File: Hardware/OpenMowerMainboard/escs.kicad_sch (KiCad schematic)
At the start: 3 parts, among them U4 xESC2, U5 xESC2, U6 xESC2

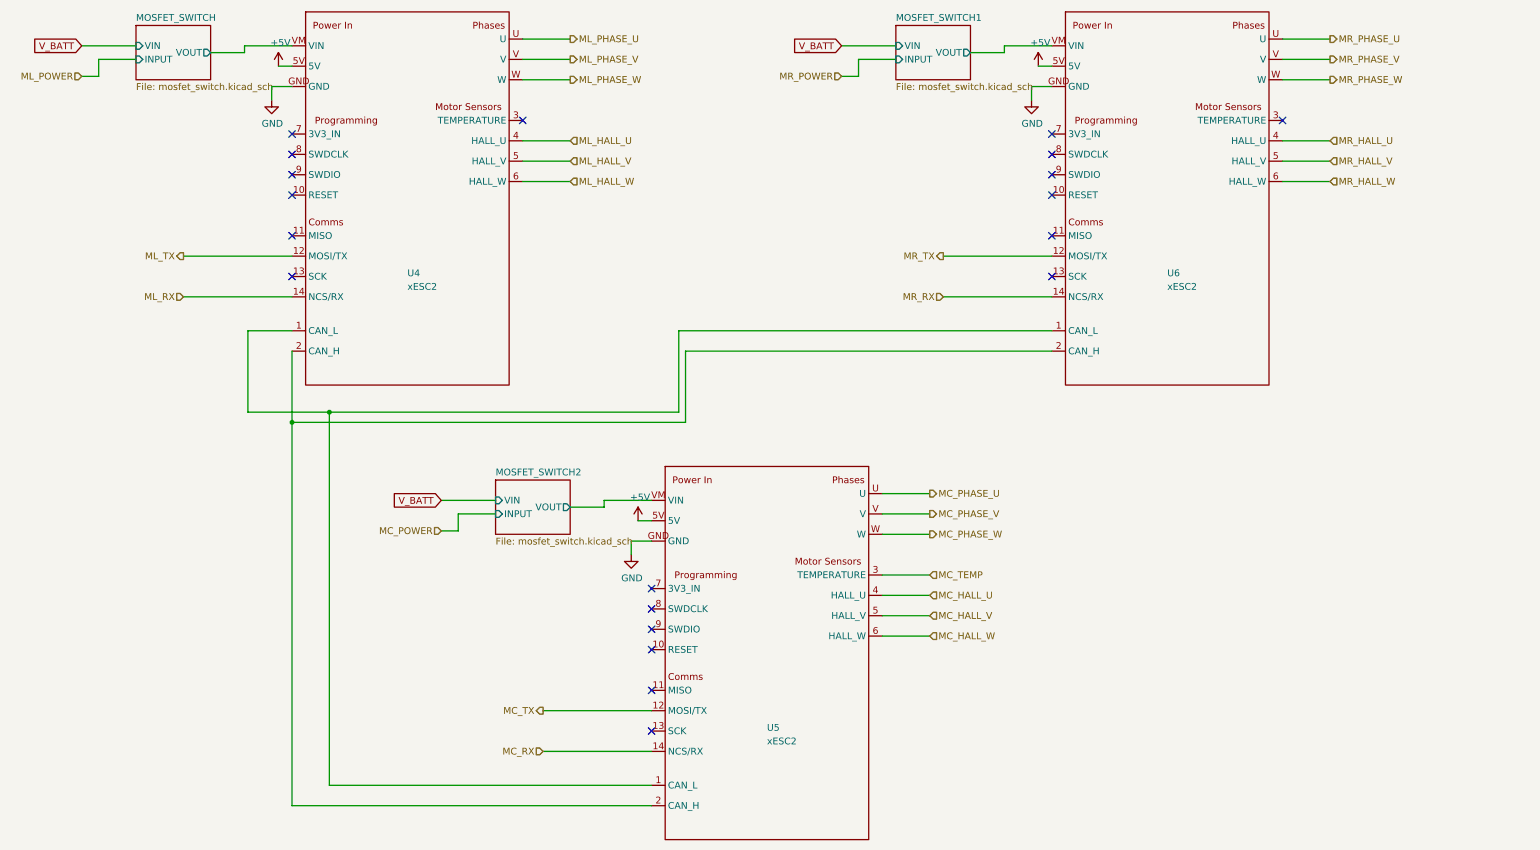
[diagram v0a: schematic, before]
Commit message: wip schematic
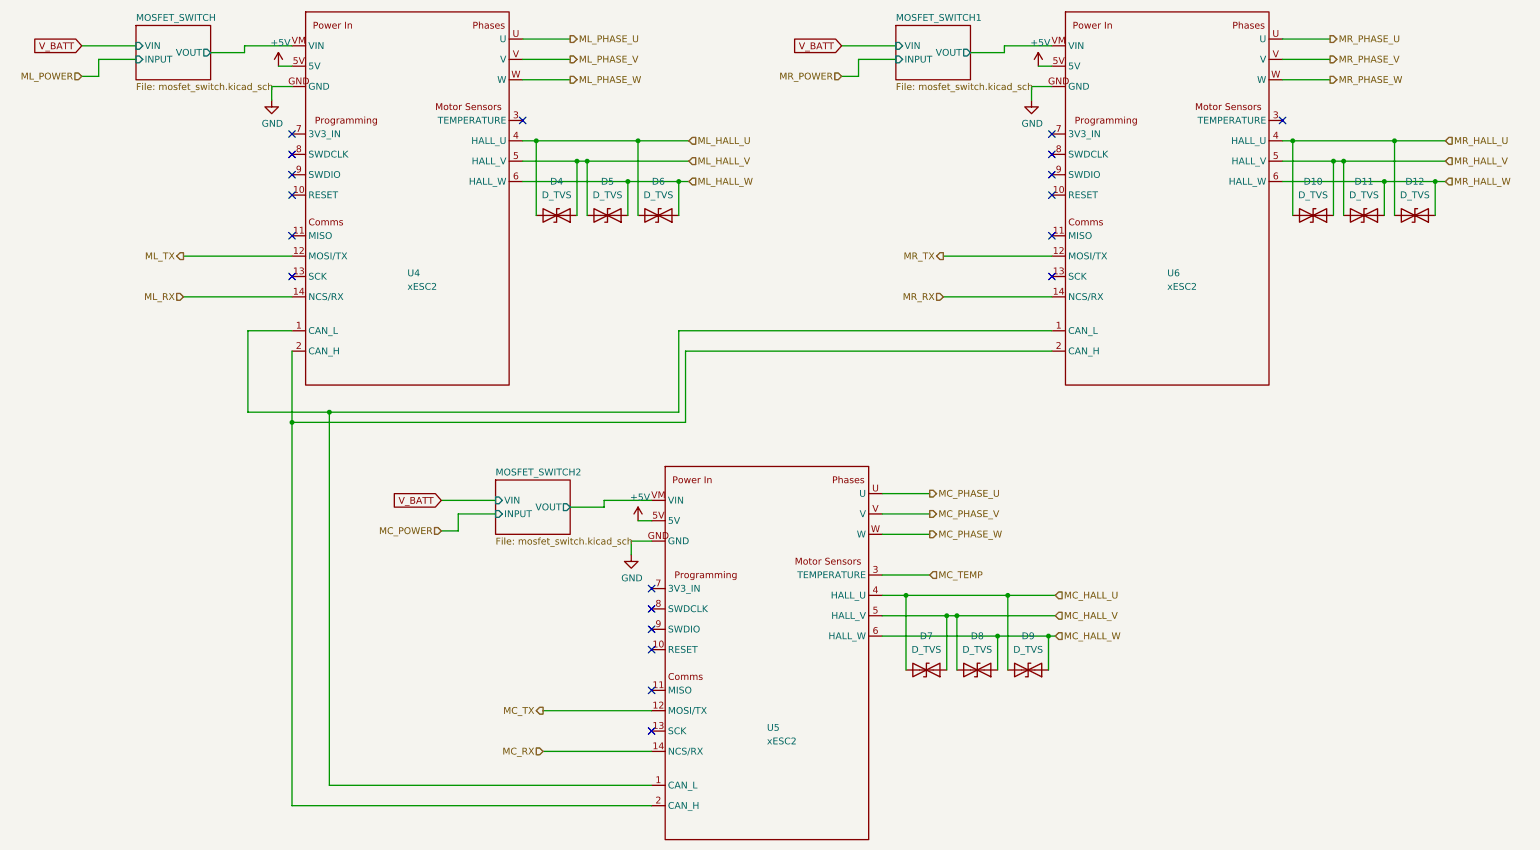
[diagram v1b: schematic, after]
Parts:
- added D10, D11, D12, D4, D5, D6, D7, D8, D9: D_TVS, Diode_SMD:D_SMB, symbol Device:D_TVS
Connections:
- net MC_HALL_U: now also D7.2 (A2), D9.2 (A2)
- net MC_HALL_V: now also D7.1 (A1), D8.2 (A2)
- net MC_HALL_W: now also D8.1 (A1), D9.1 (A1)
- net ML_HALL_U: now also D4.2 (A2), D6.2 (A2)
- net ML_HALL_V: now also D4.1 (A1), D5.2 (A2)
- net ML_HALL_W: now also D5.1 (A1), D6.1 (A1)
- net MR_HALL_U: now also D10.2 (A2), D12.2 (A2)
- net MR_HALL_V: now also D10.1 (A1), D11.2 (A2)
- net MR_HALL_W: now also D11.1 (A1), D12.1 (A1)

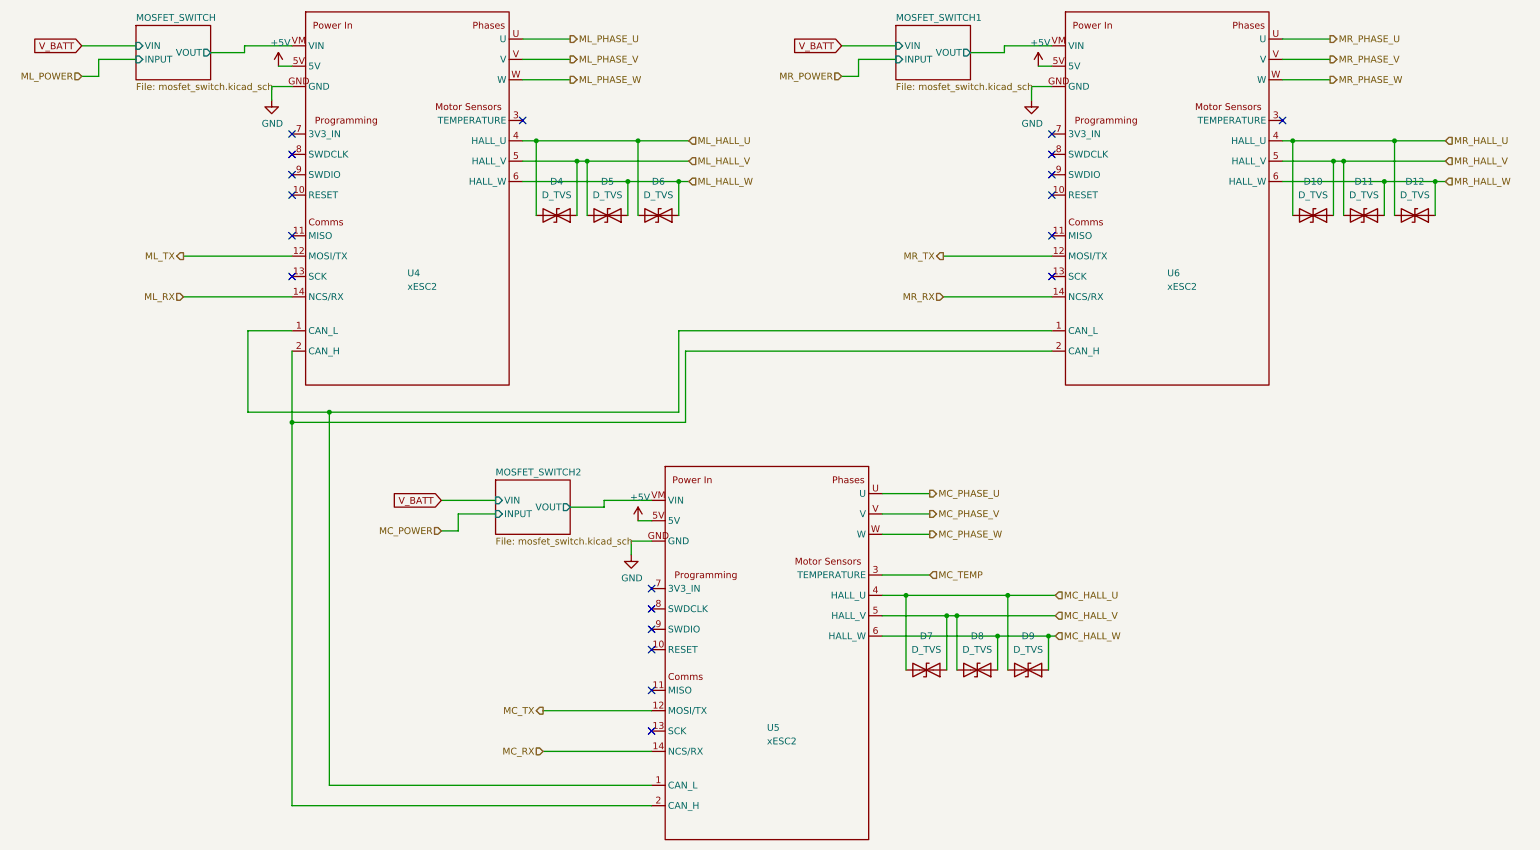
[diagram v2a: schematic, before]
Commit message: wip
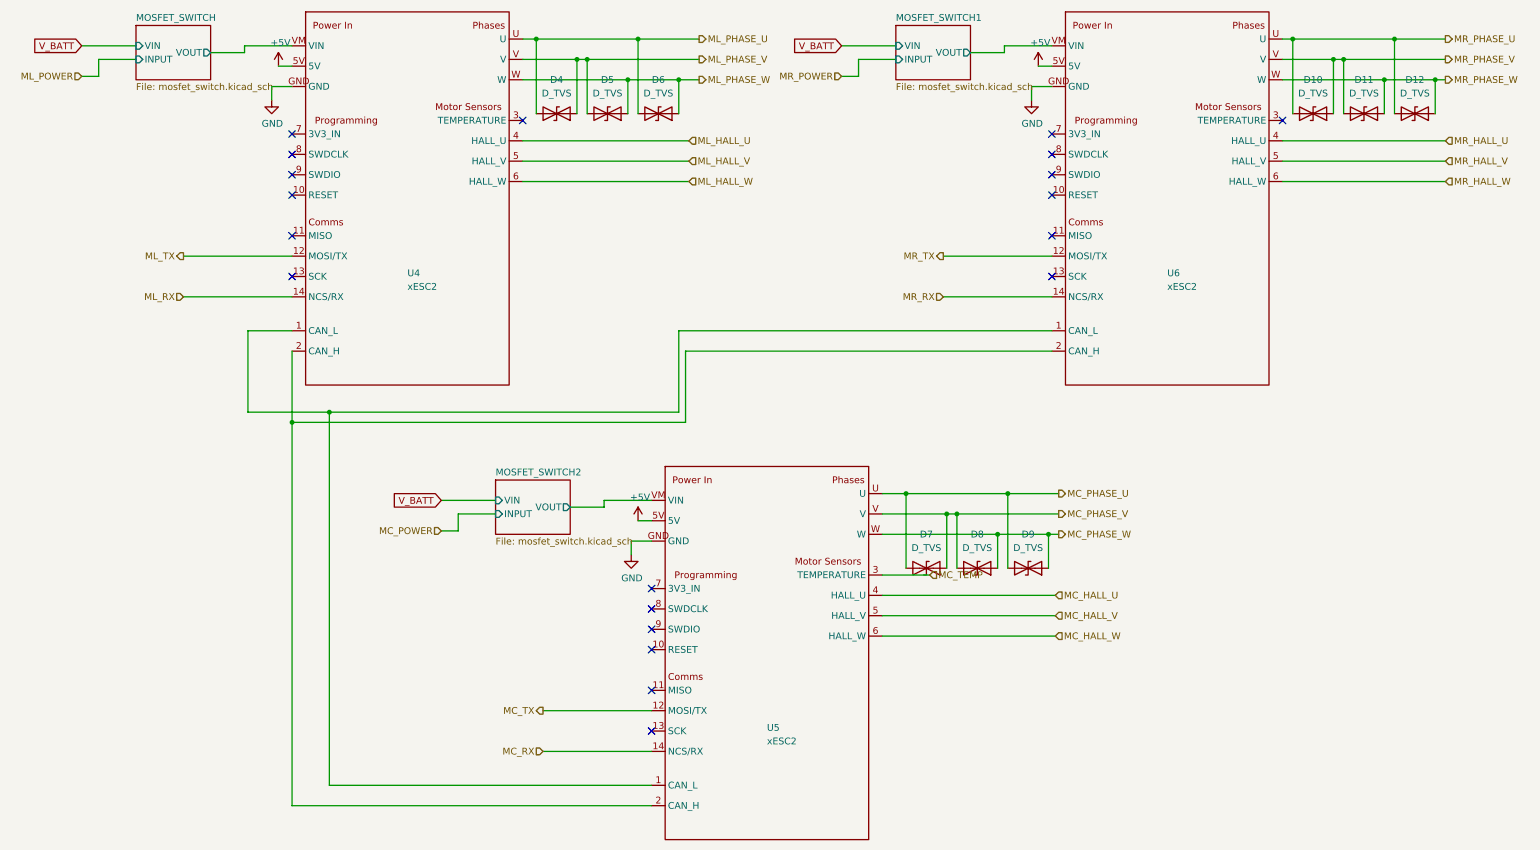
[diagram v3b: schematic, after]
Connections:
- net MC_HALL_U: no longer D7.2 (A2), D9.2 (A2)
- net MC_HALL_V: no longer D7.1 (A1), D8.2 (A2)
- net MC_HALL_W: no longer D8.1 (A1), D9.1 (A1)
- net MC_PHASE_U: now also D7.2 (A2), D9.2 (A2)
- net MC_PHASE_V: now also D7.1 (A1), D8.2 (A2)
- net MC_PHASE_W: now also D8.1 (A1), D9.1 (A1)
- net ML_HALL_U: no longer D4.2 (A2), D6.2 (A2)
- net ML_HALL_V: no longer D4.1 (A1), D5.2 (A2)
- net ML_HALL_W: no longer D5.1 (A1), D6.1 (A1)
- net ML_PHASE_U: now also D4.2 (A2), D6.2 (A2)
- net ML_PHASE_V: now also D4.1 (A1), D5.2 (A2)
- net ML_PHASE_W: now also D5.1 (A1), D6.1 (A1)
- net MR_HALL_U: no longer D10.2 (A2), D12.2 (A2)
- net MR_HALL_V: no longer D10.1 (A1), D11.2 (A2)
- net MR_HALL_W: no longer D11.1 (A1), D12.1 (A1)
- net MR_PHASE_U: now also D10.2 (A2), D12.2 (A2)
- net MR_PHASE_V: now also D10.1 (A1), D11.2 (A2)
- net MR_PHASE_W: now also D11.1 (A1), D12.1 (A1)
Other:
- moved on the sheet: D10, D11, D12, D4, D5, D6, D7, D8, D9
